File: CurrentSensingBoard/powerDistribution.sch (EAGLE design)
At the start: 31 parts, among them U1 MAX11635EEE+, U7 AP2114H-3.3TRG1

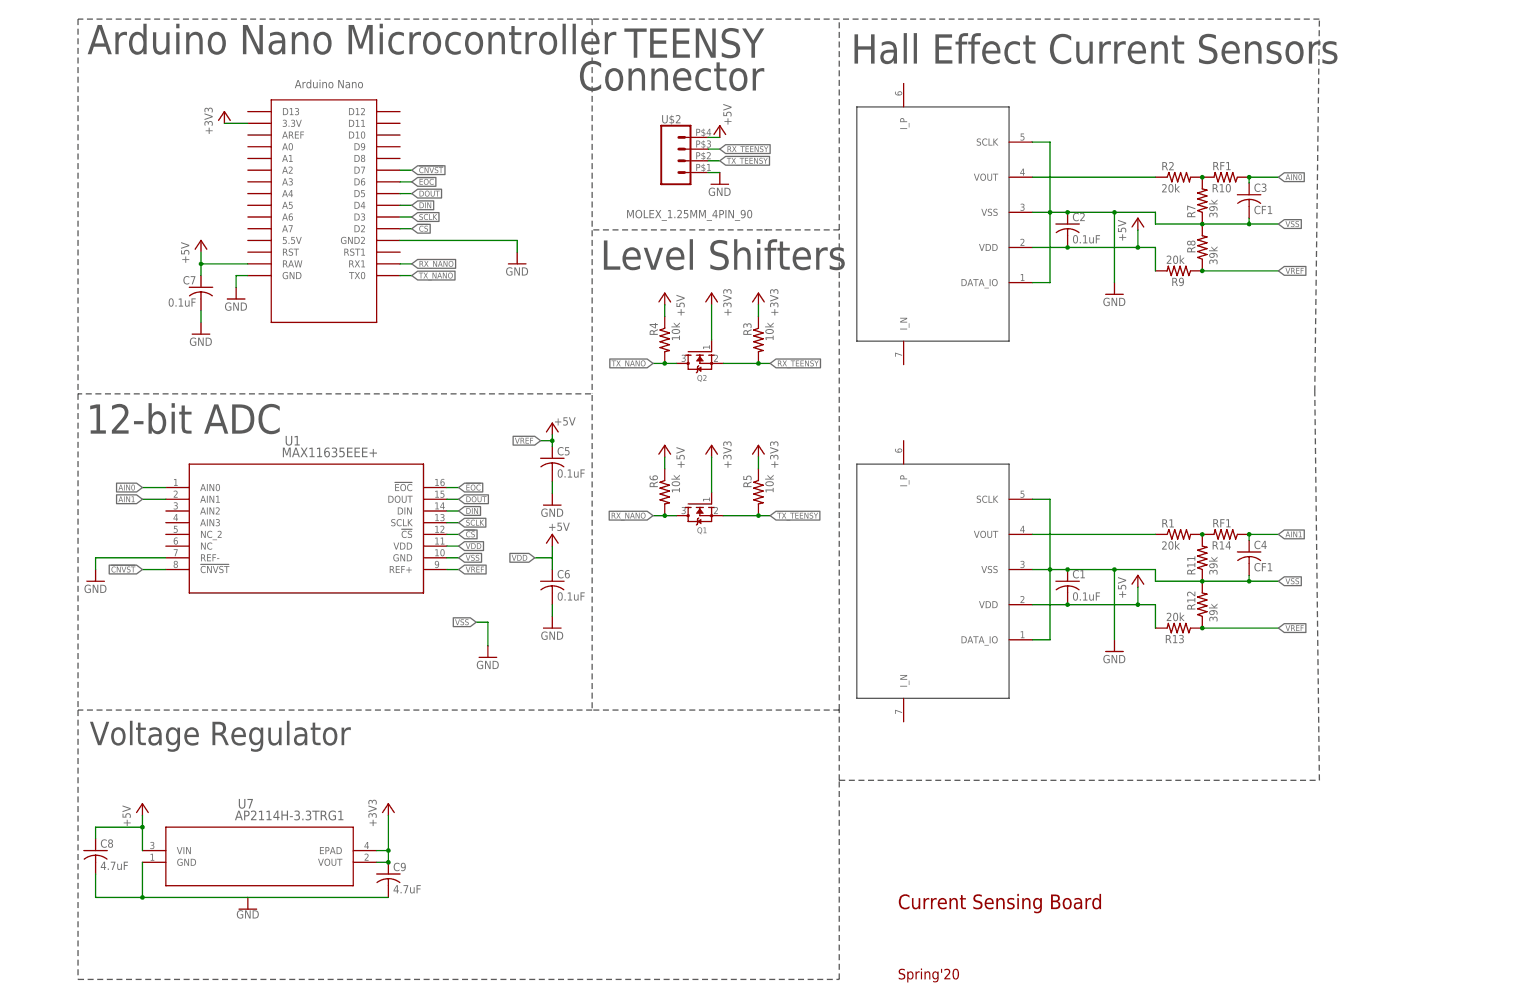
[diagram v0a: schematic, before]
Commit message: added data line connector
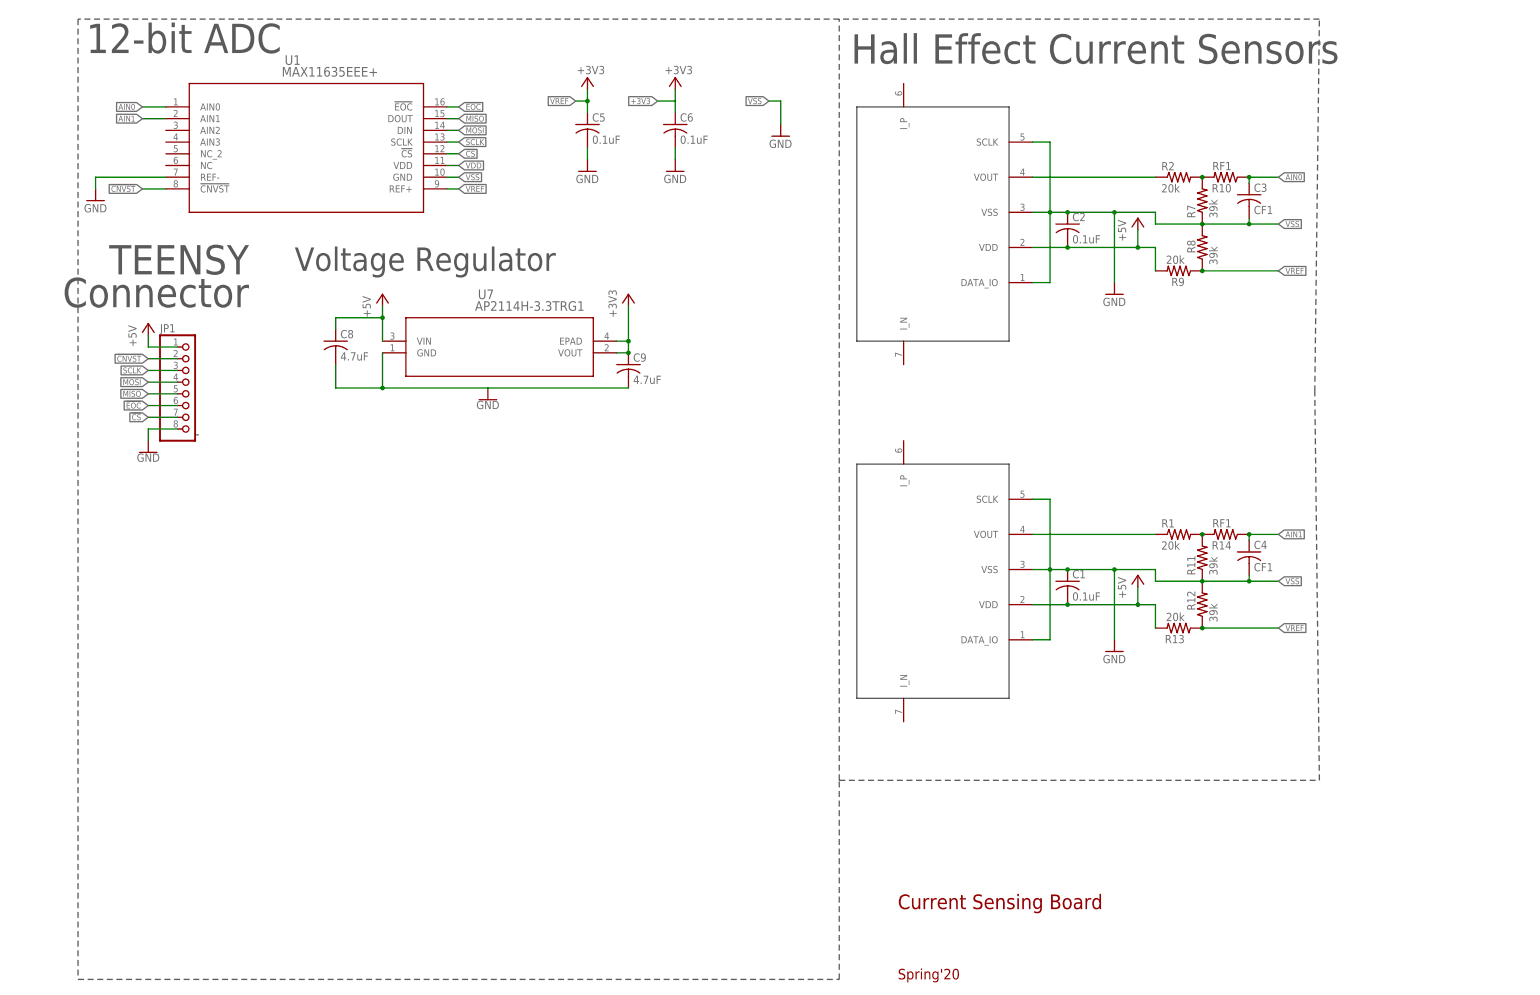
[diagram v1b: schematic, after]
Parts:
- removed C7: 0.1uF, rcl:C-USC0603
- removed Q1, Q2: (no value), Adafruit FET 4-Channel Shifter:ADAFRUIT_MOSFET-NREFLOW
- removed R3, R4, R5, R6: 10k, rcl:R-US_R0603
- removed U$1: NANO, I'mRADIOactive:NANO
- removed U$2: MOLEX_1.25MM_4PIN_90, Kirbi_ControlBoard:MOLEX_1.25MM_4PIN_90
- added JP1: (no value), pinhead:PINHD-1X8/90
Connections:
- removed net DIN: U$1.D4, U1.DIN
- removed net DOUT: U$1.D5, U1.DOUT
- removed net RX_NANO: Q1.D, R6.2, U$1.RX1
- removed net RX_TEENSY: Q2.S, R3.2, U$2.3
- removed net TX_NANO: Q2.D, R4.2, U$1.TX0
- removed net TX_TEENSY: Q1.S, R5.2, U$2.2
- new net MISO: JP1.5, U1.DOUT
- new net MOSI: JP1.4, U1.DIN
- net !CNVST!: now also JP1.2; no longer U$1.D7
- net !CS!: now also JP1.7; no longer U$1.D2
- net !EOC!: now also JP1.6; no longer U$1.D6
- net +3V3: now also C5.1, C6.1; no longer Q1.G, Q2.G, R3.1, R5.1, U$1.3.3V
- net +5V: now also JP1.1; no longer C5.1, C7.1, R4.1, R6.1, U$1.RAW, U$2.4
- net GND: now also JP1.8; no longer C7.2, U$1.GND, U$1.GND2, U$2.1
- net SCLK: now also JP1.3; no longer U$1.D3
- net VDD: no longer C6.1
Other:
- note removed: "Arduino Nano Microcontroller"
- note removed: "Level Shifters"
- moved on the sheet: C5, C6, C8, C9, U1, U7
